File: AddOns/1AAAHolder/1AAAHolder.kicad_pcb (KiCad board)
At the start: 2 copper layers, 34.5 x 50.5 mm, 53 parts, among them P1 Contacts, P2 Contacts, P6 Contacts

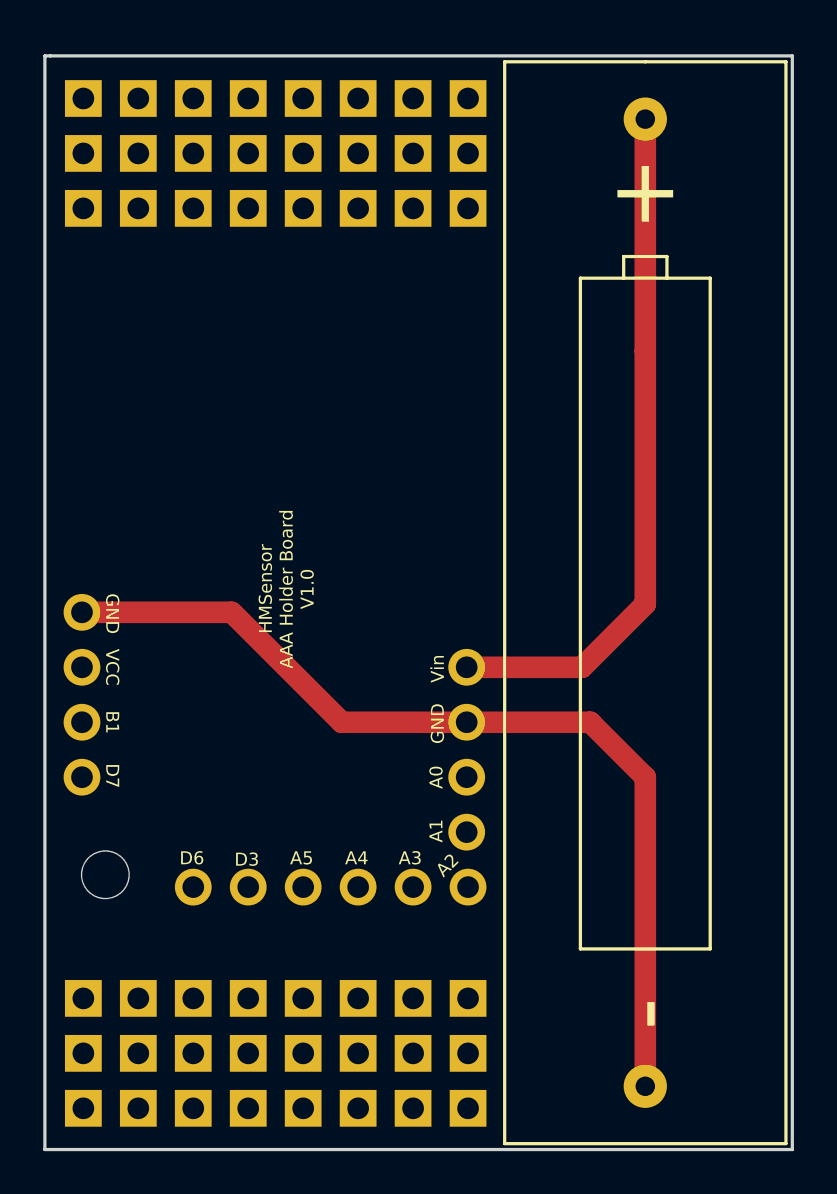
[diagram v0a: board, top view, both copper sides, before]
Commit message: panel added
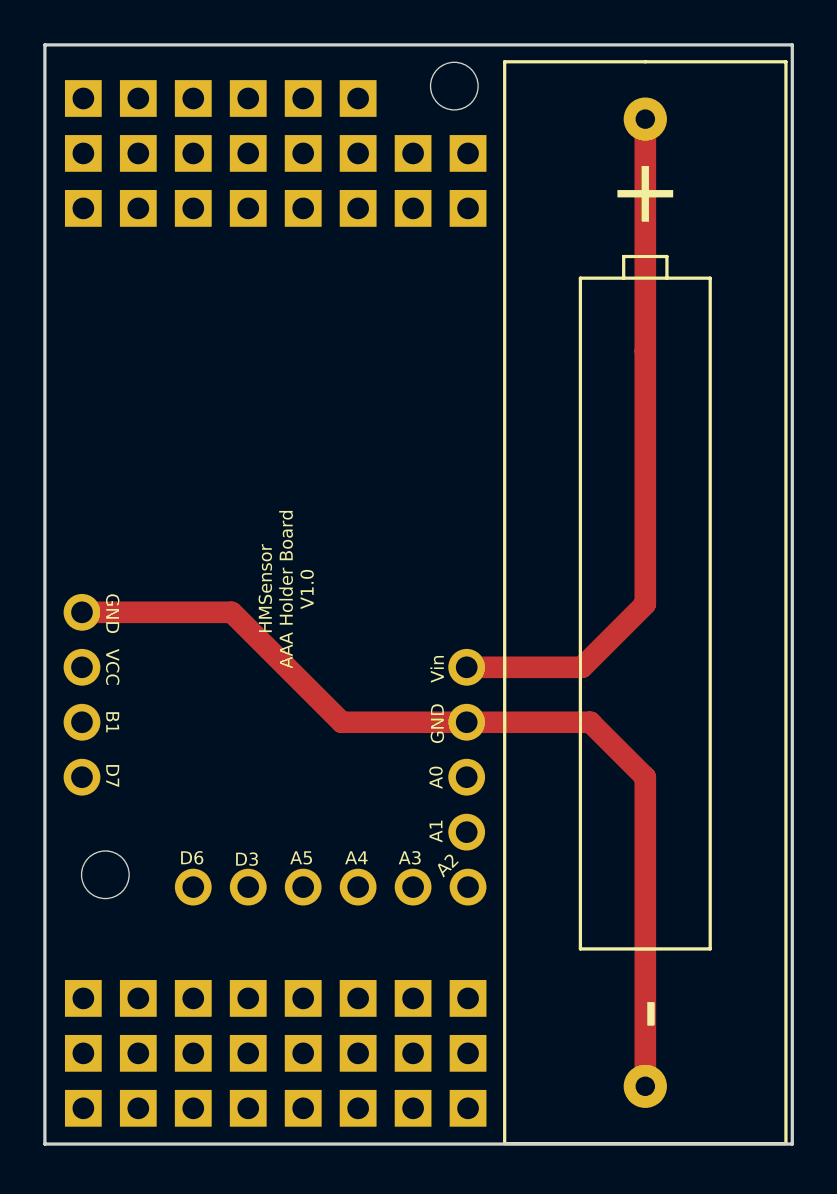
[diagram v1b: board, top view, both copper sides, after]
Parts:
- removed the REF**1 at (188.7, 87.3)
- removed the REF**2 at (186.2, 87.3)
- added REF**: MountingHole_2.2mm_M2, Mounting_Holes:MountingHole_2.2mm_M2, F.Cu at (188.1, 86.7)
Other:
- board size 34.5 x 50.5 mm -> 34.5 x 50.8 mm
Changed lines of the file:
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@@
     (links 3)
     (no_connects 0)
-    (area 169.088999 85.268999 203.783001 135.965001)
+    (area 169.088999 84.760999 203.783001 135.711001)
     (thickness 1.6)
-    (drawings 20)
+    (drawings 19)
     (tracks 10)
     (zones 0)
-    (modules 53)
+    (modules 52)
     (nets 14)
   )
@@
   )
   (setup
-    (last_trace_width 1)
+    (last_trace_width 0.25)
     (user_trace_width 1)
     (trace_clearance 0.2)
@@
     (uvia_drill 0.1)
   )
+  (module Mounting_Holes:MountingHole_2.2mm_M2 (layer F.Cu)
+    (at 188.087 86.741)
+    (descr "Mounting Hole 2.2mm, no annular, M2")
+    (tags "mounting hole 2.2mm no annular m2")
+    (fp_text reference REF** (at -0.127 4.826) (layer F.SilkS) hide
+      (effects (font (size 1 1) (thickness 0.15)))
+    )
+    (fp_text value MountingHole_2.2mm_M2 (at 0 3.2) (layer F.Fab) hide
+      (effects (font (size 1 1) (thickness 0.15)))
+    )
+    (fp_circle (center 0 0) (end 2.2 0) (layer Cmts.User) (width 0.15))
+    (fp_circle (center 0 0) (end 2.45 0) (layer F.CrtYd) (width 0.05))
+    (pad 1 np_thru_hole circle (at 0 0) (size 2.2 2.2) (drill 2.2) (layers *.Cu *.Mask))
+  )
   (module Pin_Headers:Pin_Header_Straight_1x01_Pitch2.54mm (layer F.Cu)
     (at 170.942 92.3925)
@@
     (tags "Through hole pin header THT 1x01 2.54mm single row")
     (fp_text reference REF**3 (at 0 -2.33) (layer F.SilkS) hide
-      (effects (font (size 1 1) (thickness 0.15)))
-    )
-    (fp_text value Pin_Header_Straight_1x01_Pitch2.54mm (at 0 2.33) (layer F.Fab) hide
-      (effects (font (size 1 1) (thickness 0.15)))
-    )
-    (fp_line (start -1.27 -1.27) (end -1.27 1.27) (layer F.Fab) (width 0.1))
-    (fp_line (start -1.27 1.27) (end 1.27 1.27) (layer F.Fab) (width 0.1))
-    (fp_line (start 1.27 1.27) (end 1.27 -1.27) (layer F.Fab) (width 0.1))
-    (fp_line (start 1.27 -1.27) (end -1.27 -1.27) (layer F.Fab) (width 0.1))
-    (fp_line (start -1.8 -1.8) (end -1.8 1.8) (layer F.CrtYd) (width 0.05))
-    (fp_line (start -1.8 1.8) (end 1.8 1.8) (layer F.CrtYd) (width 0.05))
-    (fp_line (start 1.8 1.8) (end 1.8 -1.8) (layer F.CrtYd) (width 0.05))
-    (fp_line (start 1.8 -1.8) (end -1.8 -1.8) (layer F.CrtYd) (width 0.05))
-    (pad 1 thru_hole rect (at 0 0) (size 1.7 1.7) (drill 1) (layers *.Cu *.Mask))
-  )
-  (module Pin_Headers:Pin_Header_Straight_1x01_Pitch2.54mm (layer F.Cu)
-    (at 186.182 87.3125)
-    (descr "Through hole straight pin header, 1x01, 2.54mm pitch, single row")
-    (tags "Through hole pin header THT 1x01 2.54mm single row")
-    (fp_text reference REF**2 (at 0 -2.33) (layer F.SilkS) hide
-      (effects (font (size 1 1) (thickness 0.15)))
-    )
-    (fp_text value Pin_Header_Straight_1x01_Pitch2.54mm (at 0 2.33) (layer F.Fab) hide
-      (effects (font (size 1 1) (thickness 0.15)))
-    )
-    (fp_line (start -1.27 -1.27) (end -1.27 1.27) (layer F.Fab) (width 0.1))
-    (fp_line (start -1.27 1.27) (end 1.27 1.27) (layer F.Fab) (width 0.1))
-    (fp_line (start 1.27 1.27) (end 1.27 -1.27) (layer F.Fab) (width 0.1))
-    (fp_line (start 1.27 -1.27) (end -1.27 -1.27) (layer F.Fab) (width 0.1))
-    (fp_line (start -1.8 -1.8) (end -1.8 1.8) (layer F.CrtYd) (width 0.05))
-    (fp_line (start -1.8 1.8) (end 1.8 1.8) (layer F.CrtYd) (width 0.05))
-    (fp_line (start 1.8 1.8) (end 1.8 -1.8) (layer F.CrtYd) (width 0.05))
-    (fp_line (start 1.8 -1.8) (end -1.8 -1.8) (layer F.CrtYd) (width 0.05))
-    (pad 1 thru_hole rect (at 0 0) (size 1.7 1.7) (drill 1) (layers *.Cu *.Mask))
-  )
-  (module Pin_Headers:Pin_Header_Straight_1x01_Pitch2.54mm (layer F.Cu)
-    (at 188.722 87.3125)
-    (descr "Through hole straight pin header, 1x01, 2.54mm pitch, single row")
-    (tags "Through hole pin header THT 1x01 2.54mm single row")
-    (fp_text reference REF**1 (at 0 -2.33) (layer F.SilkS) hide
       (effects (font (size 1 1) (thickness 0.15)))
     )
@@
     )
   )
-  (gr_line (start 169.164 85.344) (end 169.418 85.344) (angle 90) (layer Edge.Cuts) (width 0.15))
-  (gr_line (start 169.164 135.89) (end 203.708 135.89) (angle 90) (layer Edge.Cuts) (width 0.15))
-  (gr_line (start 169.164 85.344) (end 169.164 135.89) (angle 90) (layer Edge.Cuts) (width 0.15))
-  (gr_line (start 203.708 85.344) (end 203.708 135.89) (angle 90) (layer Edge.Cuts) (width 0.15))
-  (gr_line (start 169.418 85.344) (end 203.708 85.344) (angle 90) (layer Edge.Cuts) (width 0.15))
+  (gr_line (start 169.164 135.636) (end 169.164 84.836) (angle 90) (layer Edge.Cuts) (width 0.15))
+  (gr_line (start 203.708 135.636) (end 203.708 84.836) (angle 90) (layer Edge.Cuts) (width 0.15))
+  (gr_line (start 169.164 135.636) (end 203.708 135.636) (angle 90) (layer Edge.Cuts) (width 0.15))
+  (gr_line (start 169.164 84.836) (end 203.708 84.836) (angle 90) (layer Edge.Cuts) (width 0.15))
   (gr_text D7 (at 172.2755 118.618 270) (layer F.SilkS)
     (effects (font (size 0.6 0.6) (thickness 0.1)))
